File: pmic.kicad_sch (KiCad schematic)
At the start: 1 part, among them U2 MP5470GL-0000-P

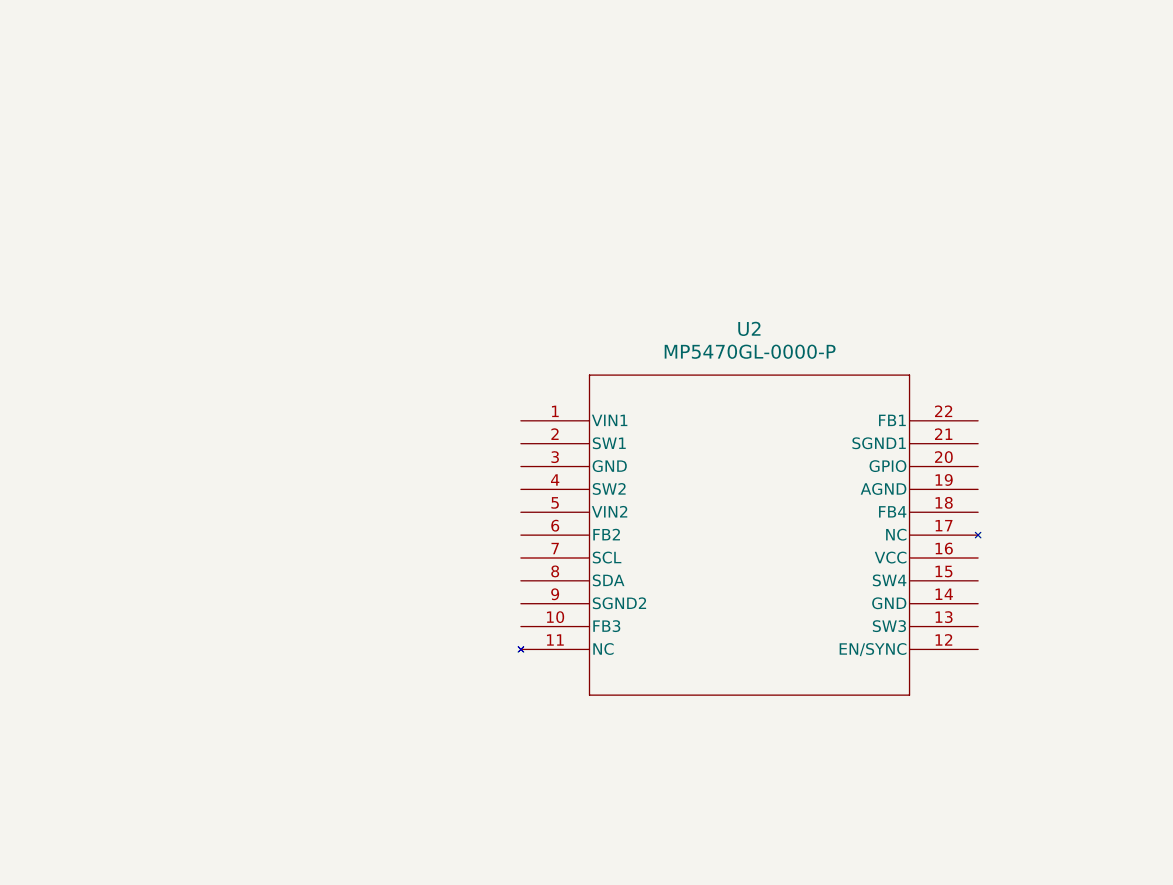
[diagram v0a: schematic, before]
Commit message: more stuff!
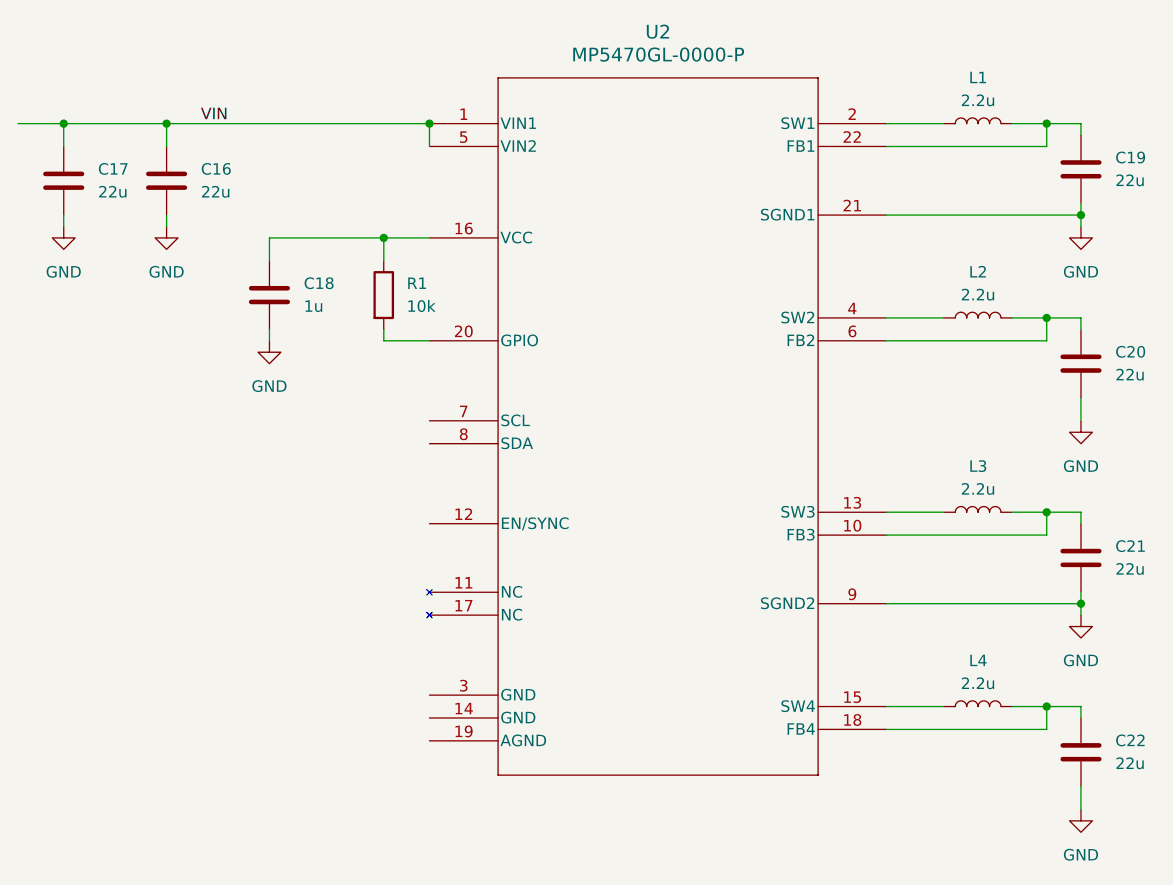
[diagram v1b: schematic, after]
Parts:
- added C16, C17, C19, C20, C21, C22: 22u, Capacitor_SMD:C_0603_1608Metric, symbol Device:C
- added C18: 1u, Capacitor_SMD:C_0402_1005Metric, symbol Device:C
- added L1, L2, L3, L4: 2.2u, Inductor_SMD:L_Bourns-SRN4018, symbol Device:L
- added R1: 10k, Resistor_SMD:R_0402_1005Metric, symbol Device:R
- U2: footprint QFN-3x4_MP5470_MNP -> MP5470:QFN-3x4_MP5470_MNP
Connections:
- net VIN: now reaches U2.1 (VIN1)
- net VIN: now also U2.5 (VIN2), C16.1, C17.1
- net at U2.10 (FB3): now also C21.1, L3.2
- net at U2.13 (SW3): now also L3.1
- net at U2.15 (SW4): now also L4.1
- net at U2.16 (VCC): now also C18.1, R1.1
- net at U2.18 (FB4): now also C22.1, L4.2
- net at U2.2 (SW1): now also L1.1
- net at U2.20 (GPIO): now also R1.2
- net GND: now reaches U2.21 (SGND1)
- net GND: now also U2.9 (SGND2), C16.2, C17.2, C18.2, C19.2, C20.2, C21.2, C22.2
- net at U2.22 (FB1): now also C19.1, L1.2
- net at U2.4 (SW2): now also L2.1
- net at U2.6 (FB2): now also C20.1, L2.2
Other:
- moved on the sheet: U2
